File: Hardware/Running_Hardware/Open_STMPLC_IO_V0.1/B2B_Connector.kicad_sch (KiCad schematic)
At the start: 41 parts, among them J1 Screw_Terminal_01x10, J2 Screw_Terminal_01x06, J39 10144517-041802LF, J41 10144517-041802LF, J42 10144517-041802LF, J43 Screw_Terminal_01x02, J9 DE9_Pins, Q5 AOD407, Q6 AOD407, Q7 MMBT5401

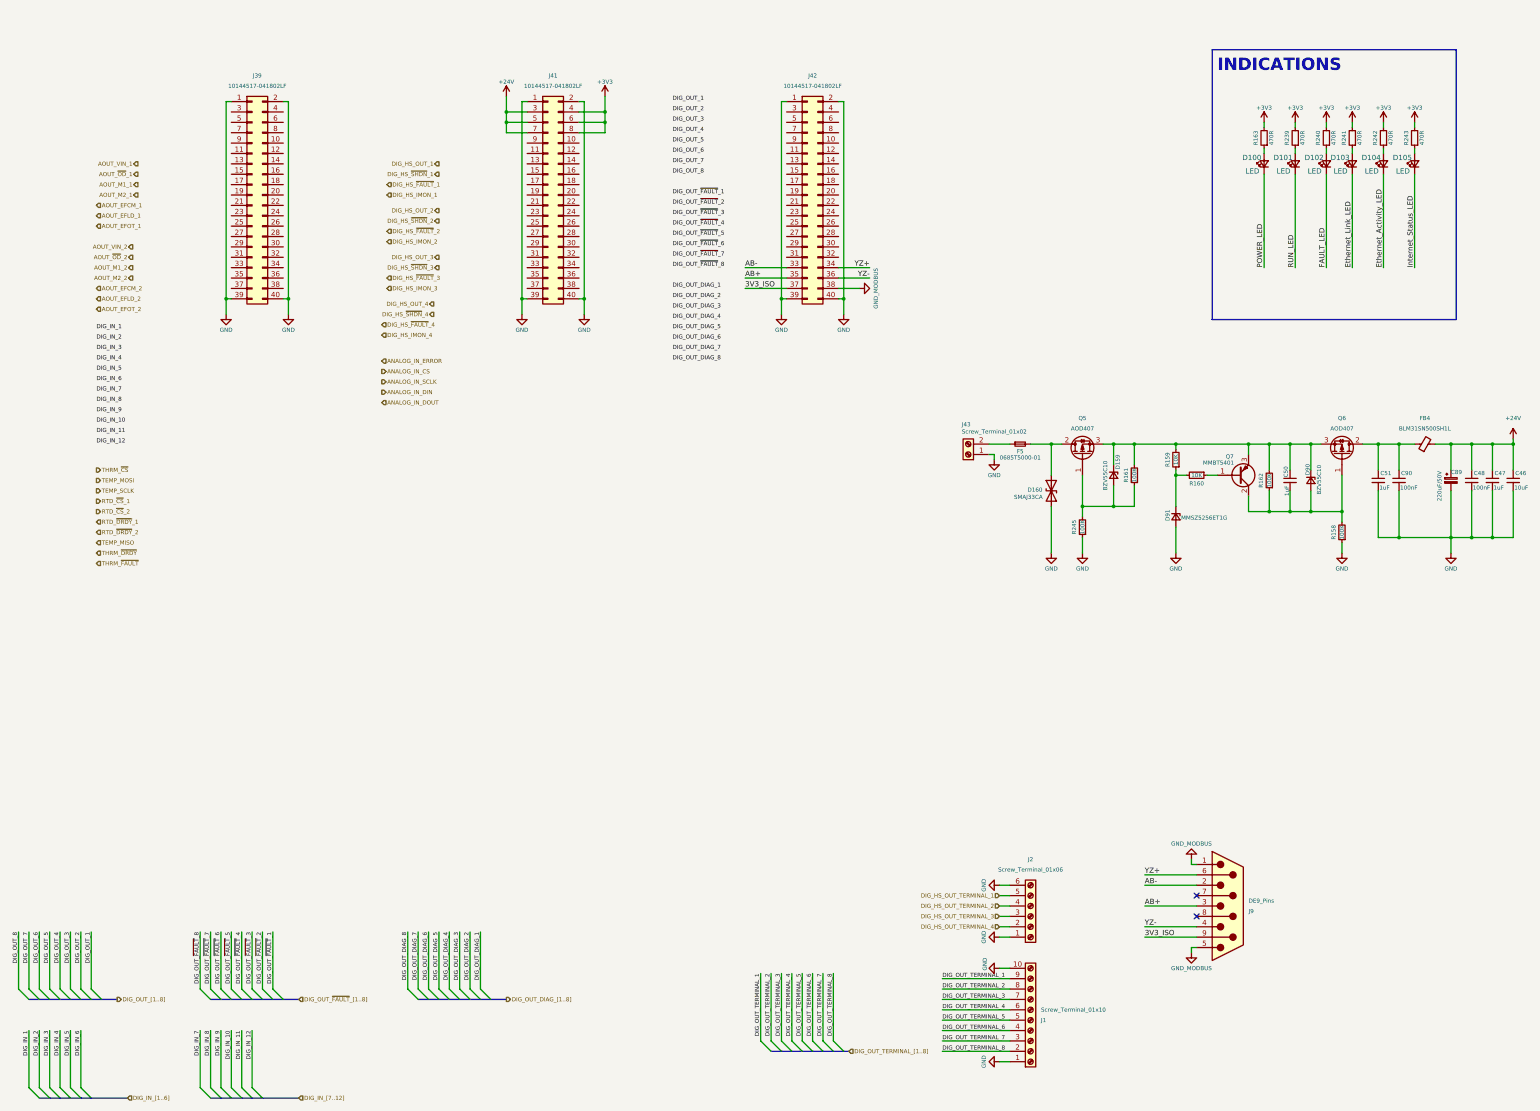
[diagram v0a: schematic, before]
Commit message: IO board layout
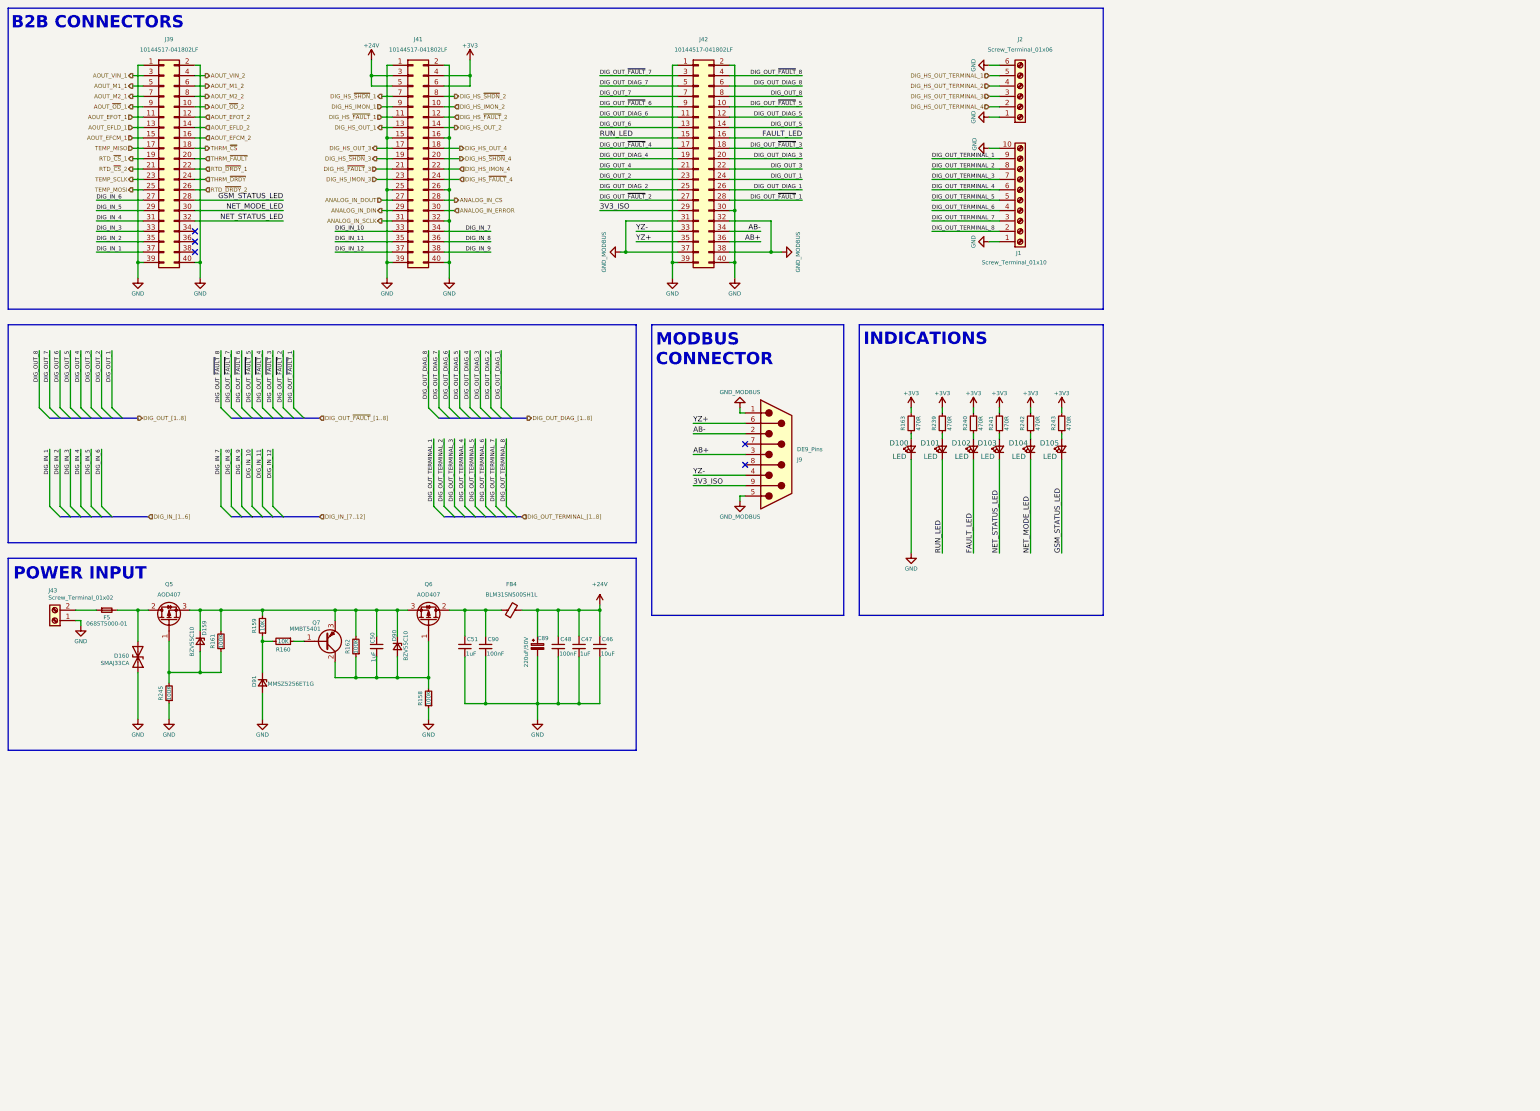
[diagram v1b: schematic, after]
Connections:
- net Ethernet_Activity_LED is gone; now on net NET_MODE_LED: D104.1 (K)
- net Ethernet_Link_LED is gone; now on net NET_STATUS_LED: D103.1 (K)
- net Internet_Status_LED is gone; now on net GSM_STATUS_LED: D105.1 (K)
- net POWER_LED is gone; now on net GND: D100.1 (K)
- net +24V: no longer J41.7 (Pin_7)
- net +3V3: no longer J41.8 (Pin_8)
- net 3V3_ISO: now also J42.29 (Pin_29); no longer J42.37 (Pin_37)
- net AB+: now also J42.36 (Pin_36); no longer J42.35 (Pin_35)
- net AB-: now also J42.34 (Pin_34); no longer J42.33 (Pin_33)
- net ANALOG_IN_CS: now also J41.28 (Pin_28)
- net ANALOG_IN_DIN: now also J41.29 (Pin_29)
- net ANALOG_IN_DOUT: now also J41.27 (Pin_27)
- net ANALOG_IN_ERROR: now also J41.30 (Pin_30)
- net ANALOG_IN_SCLK: now also J41.31 (Pin_31)
- net AOUT_EFCM_1: now also J39.15 (Pin_15)
- net AOUT_EFCM_2: now also J39.16 (Pin_16)
- net AOUT_EFLD_1: now also J39.13 (Pin_13)
- net AOUT_EFLD_2: now also J39.14 (Pin_14)
- net AOUT_EFOT_1: now also J39.11 (Pin_11)
- net AOUT_EFOT_2: now also J39.12 (Pin_12)
- net AOUT_M1_1: now also J39.5 (Pin_5)
- net AOUT_M1_2: now also J39.6 (Pin_6)
- net AOUT_M2_1: now also J39.7 (Pin_7)
- net AOUT_M2_2: now also J39.8 (Pin_8)
- net AOUT_VIN_1: now also J39.3 (Pin_3)
- net AOUT_VIN_2: now also J39.4 (Pin_4)
- net AOUT_~{OD}_1: now also J39.9 (Pin_9)
- net AOUT_~{OD}_2: now also J39.10 (Pin_10)
- net DIG_HS_IMON_1: now also J41.9 (Pin_9)
- net DIG_HS_IMON_2: now also J41.10 (Pin_10)
- net DIG_HS_IMON_3: now also J41.23 (Pin_23)
- net DIG_HS_IMON_4: now also J41.22 (Pin_22)
- net DIG_HS_OUT_1: now also J41.13 (Pin_13)
- net DIG_HS_OUT_2: now also J41.14 (Pin_14)
- net DIG_HS_OUT_3: now also J41.17 (Pin_17)
- net DIG_HS_OUT_4: now also J41.18 (Pin_18)
- net DIG_HS_~{FAULT}_1: now also J41.11 (Pin_11)
- net DIG_HS_~{FAULT}_2: now also J41.12 (Pin_12)
- net DIG_HS_~{FAULT}_3: now also J41.21 (Pin_21)
- net DIG_HS_~{FAULT}_4: now also J41.24 (Pin_24)
- net DIG_HS_~{SHDN}_1: now also J41.7 (Pin_7)
- net DIG_HS_~{SHDN}_2: now also J41.8 (Pin_8)
- net DIG_HS_~{SHDN}_3: now also J41.19 (Pin_19)
- net DIG_HS_~{SHDN}_4: now also J41.20 (Pin_20)
- net DIG_IN_1: now also J39.37 (Pin_37)
- net DIG_IN_10: now also J41.33 (Pin_33)
- net DIG_IN_11: now also J41.35 (Pin_35)
- net DIG_IN_12: now also J41.37 (Pin_37)
- net DIG_IN_2: now also J39.35 (Pin_35)
- net DIG_IN_3: now also J39.33 (Pin_33)
- net DIG_IN_4: now also J39.31 (Pin_31)
- net DIG_IN_5: now also J39.29 (Pin_29)
- net DIG_IN_6: now also J39.27 (Pin_27)
- net DIG_IN_7: now also J41.34 (Pin_34)
- net DIG_IN_8: now also J41.36 (Pin_36)
- net DIG_IN_9: now also J41.38 (Pin_38)
- net DIG_OUT_1: now also J42.24 (Pin_24)
- net DIG_OUT_2: now also J42.23 (Pin_23)
- net DIG_OUT_3: now also J42.22 (Pin_22)
- net DIG_OUT_4: now also J42.21 (Pin_21)
- net DIG_OUT_5: now also J42.14 (Pin_14)
- net DIG_OUT_6: now also J42.13 (Pin_13)
- net DIG_OUT_7: now also J42.7 (Pin_7)
- net DIG_OUT_8: now also J42.8 (Pin_8)
- net DIG_OUT_DIAG_1: now also J42.26 (Pin_26)
- net DIG_OUT_DIAG_2: now also J42.25 (Pin_25)
- net DIG_OUT_DIAG_3: now also J42.20 (Pin_20)
- net DIG_OUT_DIAG_4: now also J42.19 (Pin_19)
- net DIG_OUT_DIAG_5: now also J42.12 (Pin_12)
- net DIG_OUT_DIAG_6: now also J42.11 (Pin_11)
- net DIG_OUT_DIAG_7: now also J42.5 (Pin_5)
- net DIG_OUT_DIAG_8: now also J42.6 (Pin_6)
- net DIG_OUT_~{FAULT}_1: now also J42.28 (Pin_28)
- net DIG_OUT_~{FAULT}_2: now also J42.27 (Pin_27)
- net DIG_OUT_~{FAULT}_3: now also J42.18 (Pin_18)
- net DIG_OUT_~{FAULT}_4: now also J42.17 (Pin_17)
- net DIG_OUT_~{FAULT}_5: now also J42.10 (Pin_10)
- net DIG_OUT_~{FAULT}_6: now also J42.9 (Pin_9)
- net DIG_OUT_~{FAULT}_7: now also J42.3 (Pin_3)
- net DIG_OUT_~{FAULT}_8: now also J42.4 (Pin_4)
- net FAULT_LED: now also J42.16 (Pin_16)
- net GND: now also J41.15 (Pin_15), J41.16 (Pin_16), J41.25 (Pin_25), J41.26 (Pin_26), J41.32 (Pin_32), J42.30 (Pin_30)
- net GND_MODBUS: now also J42.31 (Pin_31), J42.32 (Pin_32), J42.37 (Pin_37)
- net RTD_~{CS}_1: now also J39.19 (Pin_19)
- net RTD_~{CS}_2: now also J39.21 (Pin_21)
- net RTD_~{DRDY}_1: now also J39.22 (Pin_22)
- net RTD_~{DRDY}_2: now also J39.26 (Pin_26)
- net RUN_LED: now also J42.15 (Pin_15)
- net TEMP_MISO: now also J39.17 (Pin_17)
- net TEMP_MOSI: now also J39.25 (Pin_25)
- net TEMP_SCLK: now also J39.23 (Pin_23)
- net THRM_~{CS}: now also J39.18 (Pin_18)
- net THRM_~{DRDY}: now also J39.24 (Pin_24)
- net THRM_~{FAULT}: now also J39.20 (Pin_20)
- net YZ+: now also J42.35 (Pin_35); no longer J42.34 (Pin_34)
- net YZ-: now also J42.33 (Pin_33); no longer J42.36 (Pin_36)
- net GSM_STATUS_LED: now reaches J39.28 (Pin_28)
- net NET_MODE_LED: now reaches J39.30 (Pin_30)
- net NET_STATUS_LED: now reaches J39.32 (Pin_32)
- no-connect marks 2 -> 5
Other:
- note added: "B2B CONNECTORS"
- note added: "MODBUS CONNECTOR"
- note added: "POWER INPUT"
- moved on the sheet: C46, C47, C48, C50, C51, C89, C90, D100, D101, D102, D103, D104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
